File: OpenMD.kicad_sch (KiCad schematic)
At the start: 27 parts, among them J1 GND, J2 Digital, J3 Analog, J5 A, J6 B, J7 C, J8 V_{BATT}

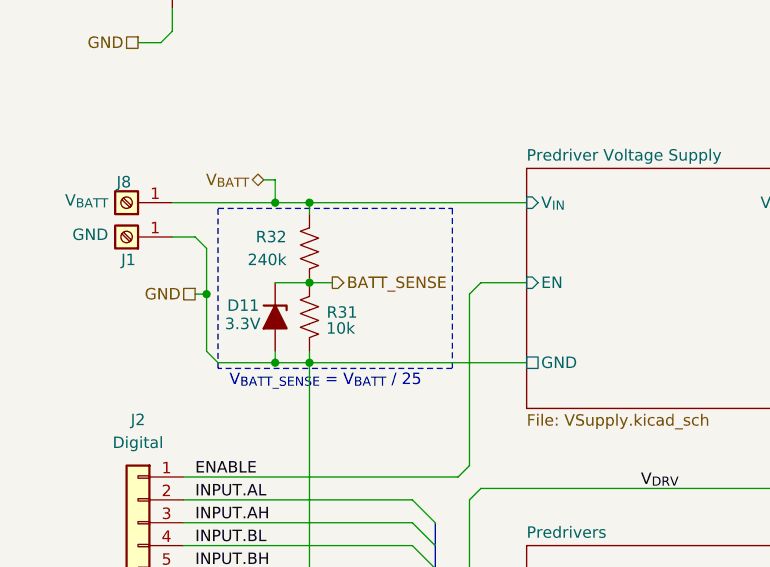
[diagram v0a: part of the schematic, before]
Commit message: revision 2
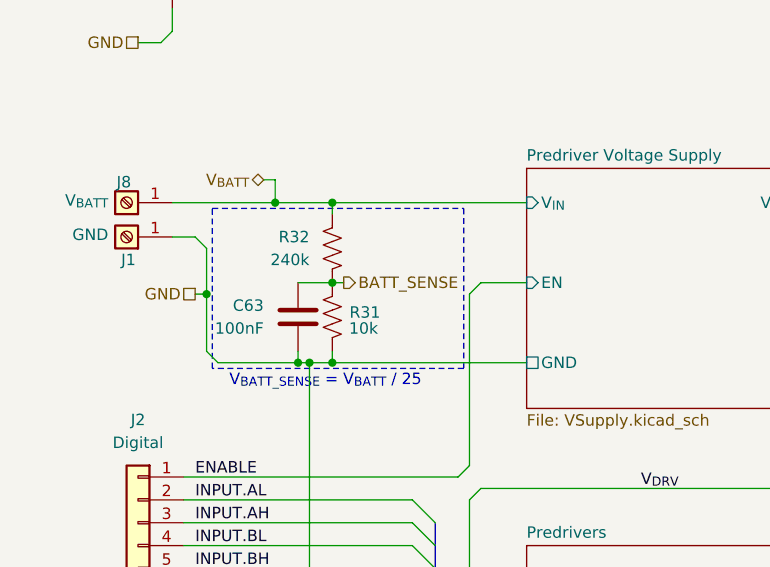
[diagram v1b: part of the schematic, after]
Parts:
- removed D11: 3.3V, Diode_SMD:D_SOD-323, symbol Device:D_Zener_Filled
- added C63: 100nF, Capacitor_SMD:C_0402_1005Metric, symbol Device:C
- C77: footprint Capacitor_SMD:C_0603_1608Metric -> Capacitor_SMD:C_0402_1005Metric; Manufacturer_Part_Number CGA0603X7R104K101JT -> (none); Rating 100V -> 5V
- R31, R32, R34, TH1: footprint Resistor_SMD:R_0603_1608Metric -> Resistor_SMD:R_0402_1005Metric
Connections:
- net BATT_SENSE: now also C63.1
- net GND: now also C63.2
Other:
- moved on the sheet: R31, R32
